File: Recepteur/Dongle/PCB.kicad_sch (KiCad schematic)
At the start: 16 parts, among them J1 USB_A, J2 Conn_01x07, J3 Conn_01x07, SW3 SW_Push, SW4 SW_Push, U1 ESP32-S3-WROOM-1, U2 MAX604, U3 ESP32-C3-WROOM-02

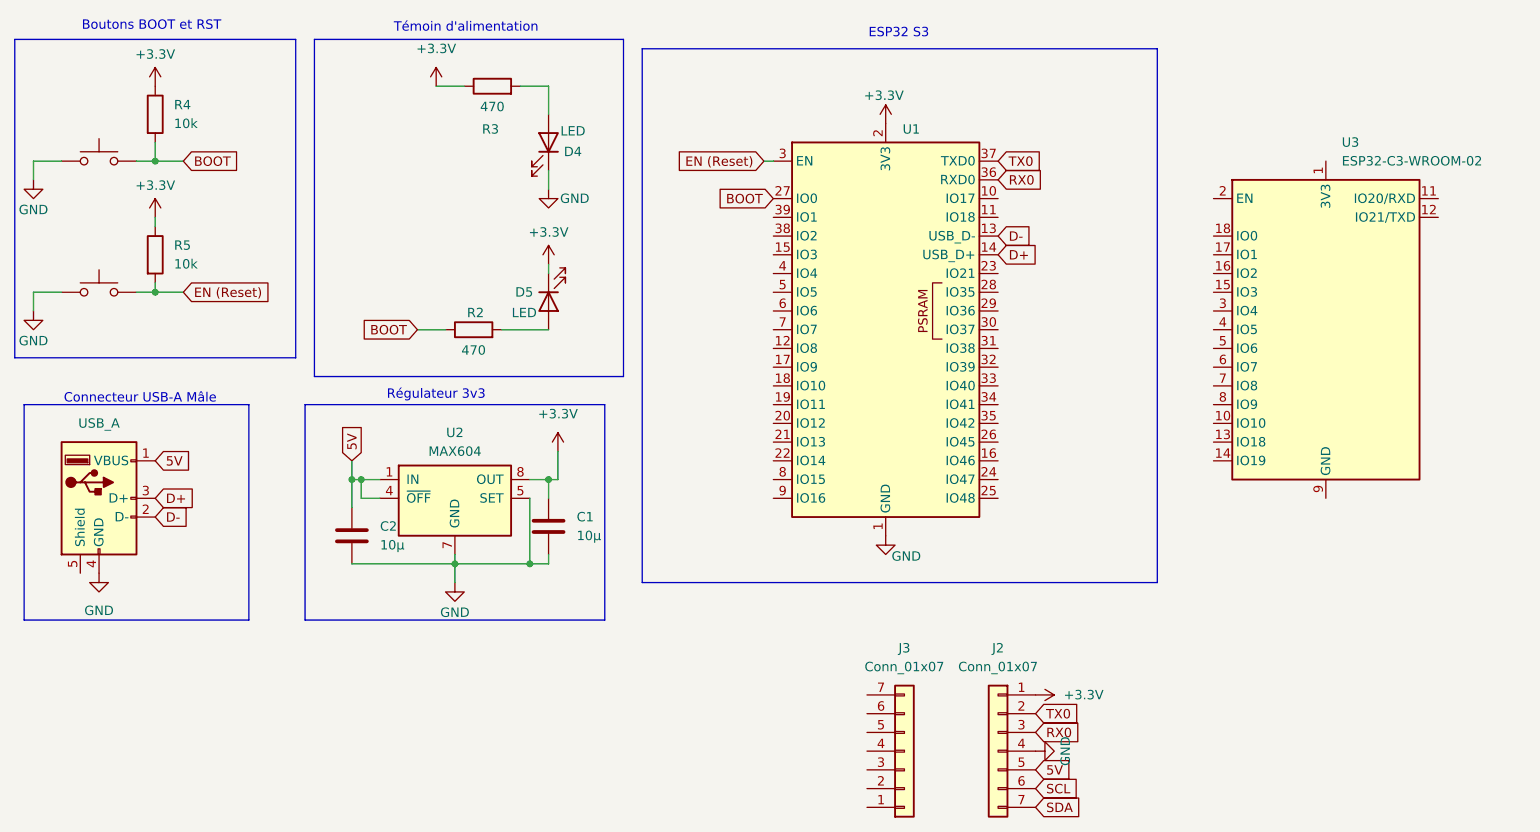
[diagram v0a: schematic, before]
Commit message: update schema & pcb
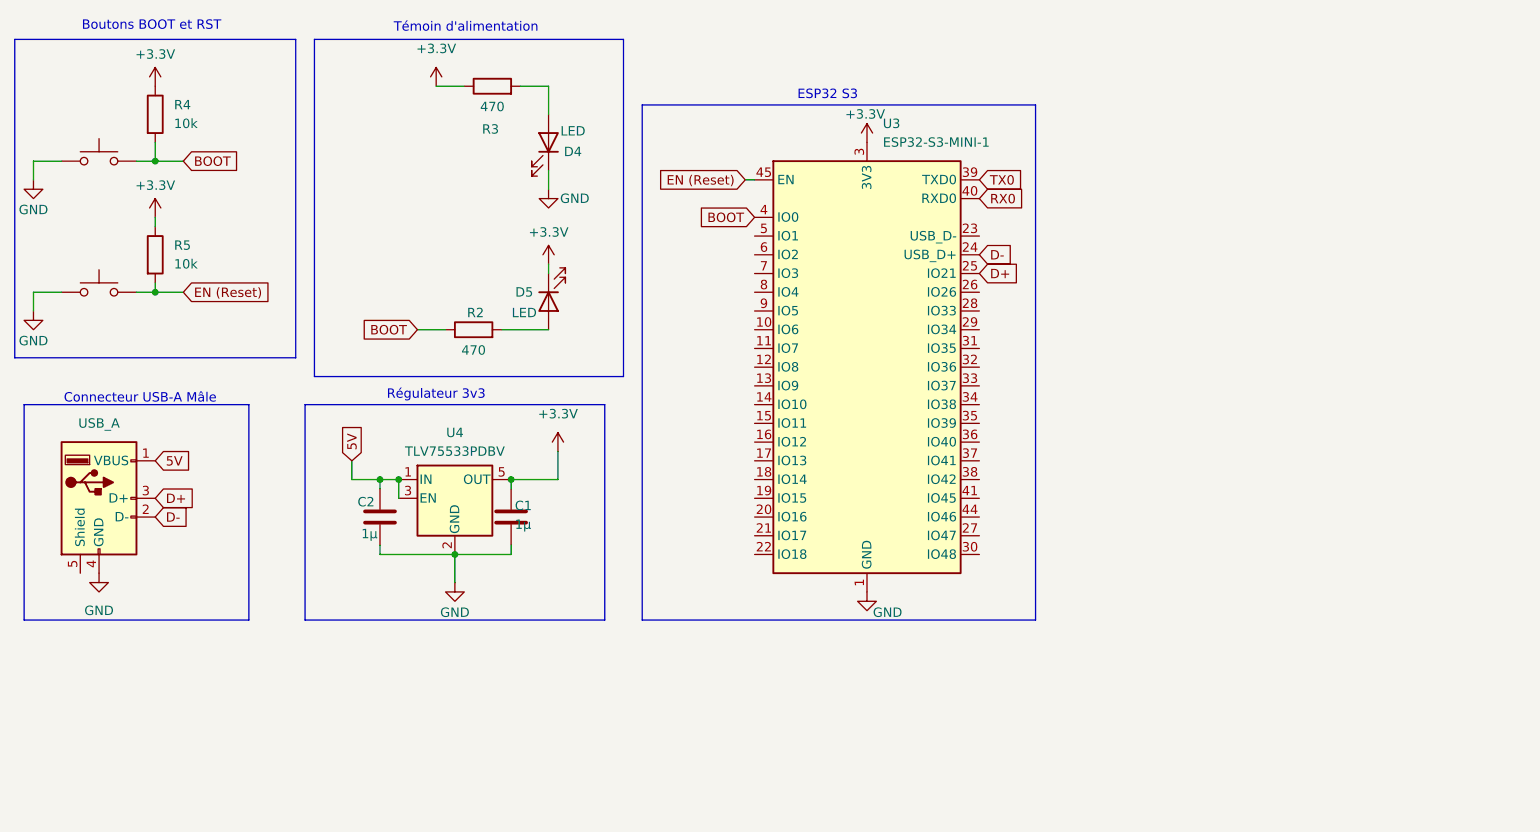
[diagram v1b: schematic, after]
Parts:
- removed J2, J3: Conn_01x07, Connector_PinHeader_2.54mm:PinHeader_1x07_P2.54mm_Vertical, symbol Connector_Generic:Conn_01x07
- removed U1: ESP32-S3-WROOM-1, RF_Module:ESP32-S3-WROOM-1, symbol RF_Module:ESP32-S3-WROOM-1
- removed U2: MAX604, Package_SO:SOIC-8-N7_3.9x4.9mm_P1.27mm, symbol Regulator_Linear:MAX604
- removed U3: ESP32-C3-WROOM-02, RF_Module:ESP32-C3-WROOM-02U, symbol RF_Module:ESP32-C3-WROOM-02
- added U3: ESP32-S3-MINI-1, RF_Module:ESP32-S2-MINI-1, symbol RF_Module:ESP32-S3-MINI-1
- added U4: TLV75533PDBV, Package_TO_SOT_SMD:SOT-23-5, symbol Regulator_Linear:TLV75533PDBV
- C1, C2: value 10µ -> 1µ
- SW3, SW4: footprint Button_Switch_SMD:Panasonic_EVQPUL_EVQPUC -> Button_Switch_SMD:SW_Tactile_SPST_NO_Straight_CK_PTS636Sx25SMTRLFS
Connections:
- net +3.3V: now also U3.3 (3V3), U4.5 (OUT)
- net 5V: now also U4.1 (IN), U4.3 (EN)
- net BOOT: now also U3.4 (IO0)
- net D+: now also U3.25 (IO21)
- net D-: now also U3.24 (USB_D+)
- net EN (Reset): now also U3.45 (EN)
- net GND: now also U3.1 (GND), U3.2 (GND), U3.42 (GND), U3.43 (GND), U3.46 (GND), U3.47 (GND), U3.48 (GND), U3.49 (GND), U3.50 (GND), U3.51 (GND), U3.52 (GND), U3.53 (GND), U3.54 (GND), U3.55 (GND), U3.56 (GND), U3.57 (GND), U3.58 (GND), U3.59 (GND), U3.60 (GND), U3.61 (GND), U3.62 (GND), U3.63 (GND), U3.64 (GND), U3.65 (GND), U4.2 (GND)
- net RX0: now also U3.40 (RXD0)
- net TX0: now also U3.39 (TXD0)
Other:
- moved on the sheet: C1, C2
